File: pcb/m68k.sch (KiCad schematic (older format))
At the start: 120 parts, among them J1 USB_B_Micro, J2 Mini-DIN-6, J4 DB15_Male_HighDensity, J5 FTSH-105-01-L-DV-K, J6 FTSH-105-01-L-DV-K, J7 FTSH-105-01-L-DV-K, J8 Micro_SD_Card, U1 93LC56, U10 25LCxxx, U11 TXB0108DQSR, U12 TXB0108DQSR, U13 iCE40-HX4K-TQ144, U14 ADV7125KSTZ50, U15 74LVC1G17, U16 LD1117S33TR_SOT223, U17 LD1117S12TR_SOT223, U18 ATL431BQDBZR, U2 68000D, U3 FT2232H, U4 TXB0108DQSR, U5 TXB0108DQSR, U6 TXB0108DQSR, U7 SN74LVC8T245PWR, U8 SN74LVC8T245PWR, U9 AS6C1616, X1 ASV-12.000MHz

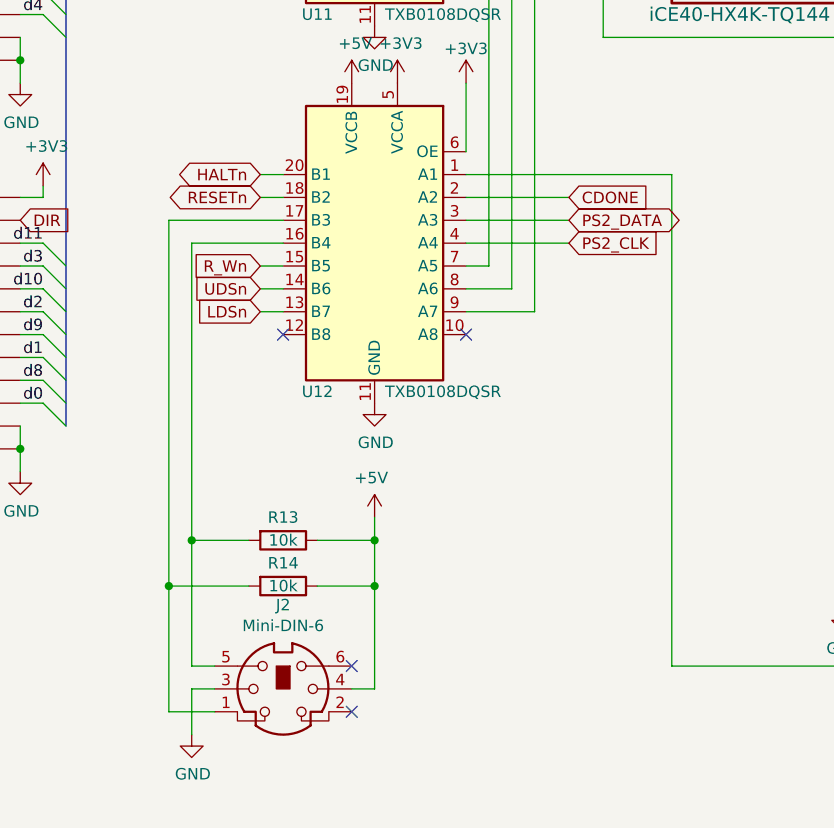
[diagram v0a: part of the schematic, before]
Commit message: Home
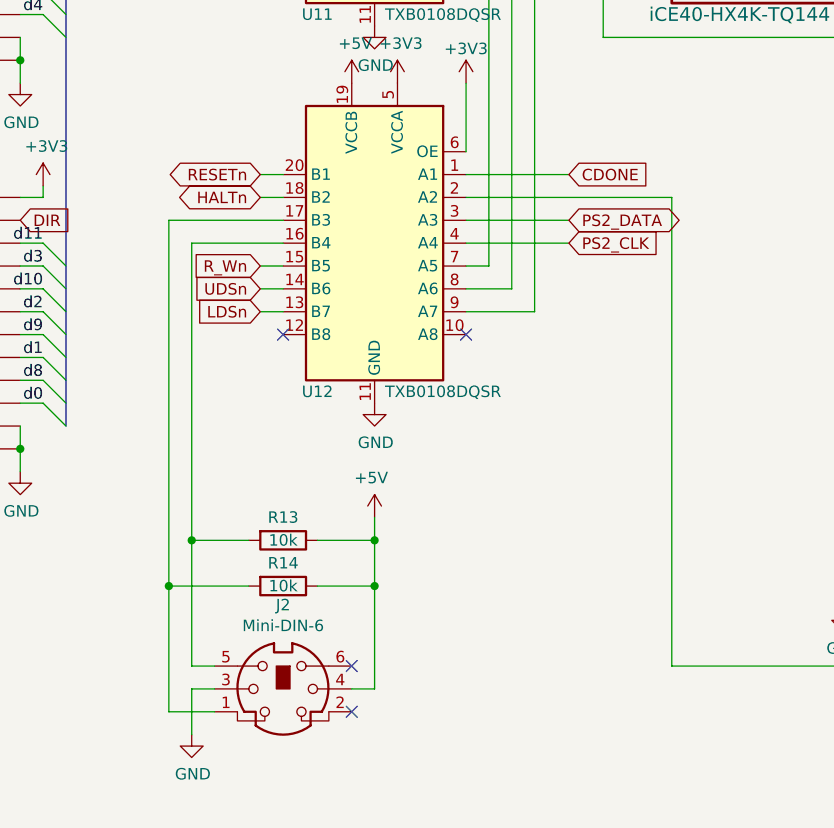
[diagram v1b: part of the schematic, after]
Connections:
- net CDONE: now also U12.1 (A1); no longer U12.2 (A2)
- net HALTn: now also U12.18 (B2); no longer U12.20 (B1)
- net RESETn: now also U12.20 (B1); no longer U12.18 (B2)
- net at U13.60 (IOB_95): now also U12.2 (A2); no longer U12.1 (A1)
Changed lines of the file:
@@
 Connection ~ 1550 14950
 Wire Wire Line
-	7050 8250 6950 8250
+	7050 8150 6950 8150
 Wire Wire Line
 	6950 7000 7050 7000
@@
 	1    0    0    -1
 $EndComp
-Text GLabel 6950 8250 0    50   BiDi ~ 0
+Text GLabel 6950 8150 0    50   BiDi ~ 0
 RESETn
-Text GLabel 8300 8250 2    50   Input ~ 0
+Text GLabel 8300 8150 2    50   Input ~ 0
 CDONE
 $Comp
@@
 Wire Wire Line
 	3400 8950 3500 8950
-Text GLabel 6950 8150 0    50   BiDi ~ 0
+Text GLabel 6950 8250 0    50   BiDi ~ 0
 HALTn
 Wire Wire Line
@@
 NoConn ~ 7050 8850
 Wire Wire Line
-	6950 8150 7050 8150
+	6950 8250 7050 8250
 Wire Wire Line
 	6550 8350 7050 8350
@@
 	7850 8350 8300 8350
 Wire Wire Line
-	7850 8250 8300 8250
-Wire Wire Line
-	7850 8150 8750 8150
+	7850 8150 8300 8150
 Wire Wire Line
-	8750 8150 8750 10300
+	7850 8250 8750 8250
 Wire Wire Line
 	8750 10300 12150 10300
@@
 Wire Wire Line
 	12150 9750 13100 9750
+Wire Wire Line
+	8750 8250 8750 10300
 Wire Bus Line
 	18600 2100 18600 2800

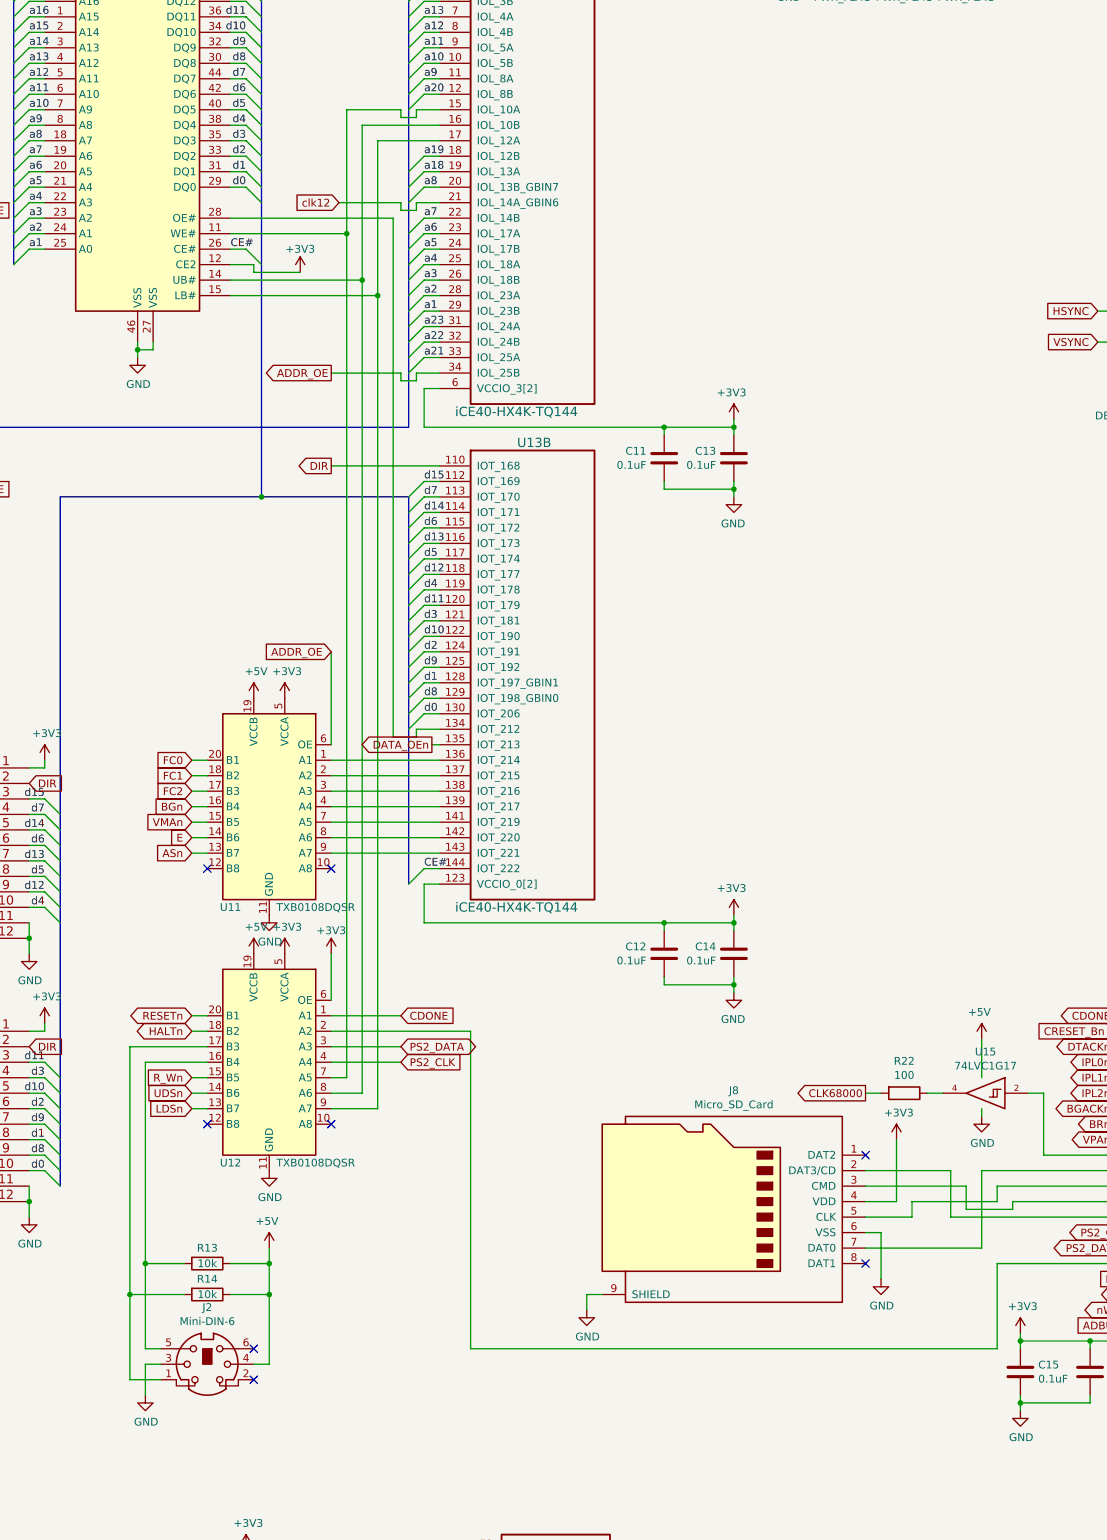
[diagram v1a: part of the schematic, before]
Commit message: I finally broke something
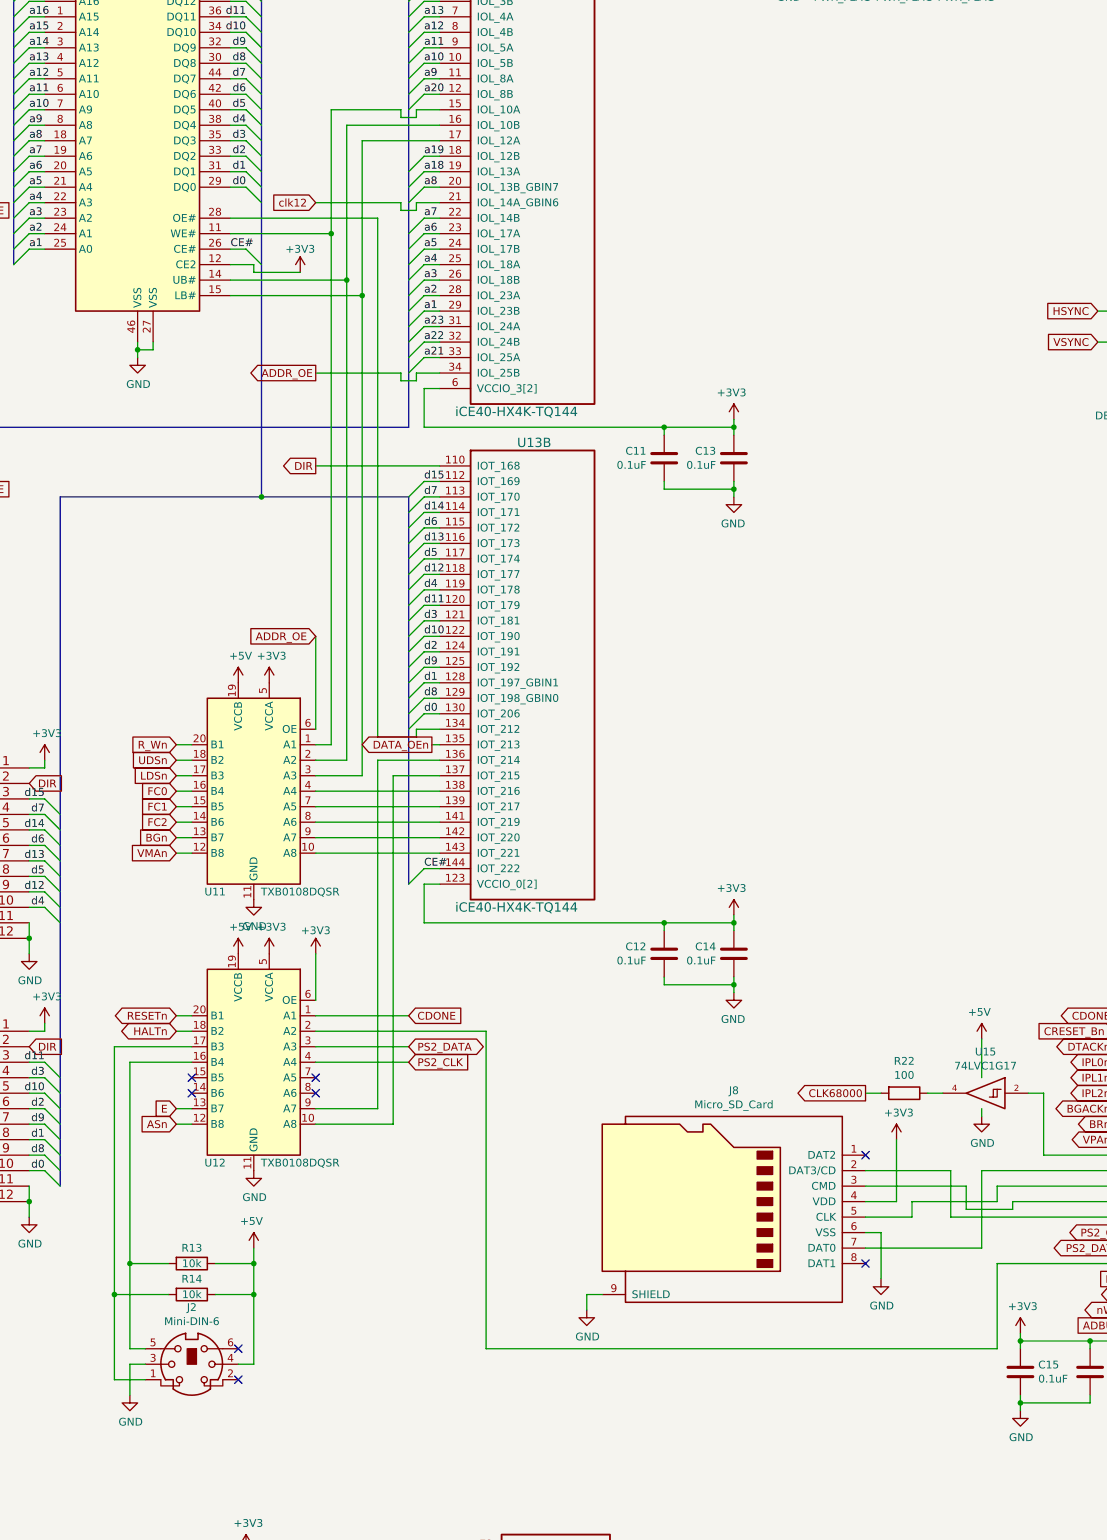
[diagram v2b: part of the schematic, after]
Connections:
- net ASn: now also U12.12 (B8); no longer U11.13 (B7)
- net BGn: now also U11.13 (B7); no longer U11.16 (B4)
- net E: now also U12.13 (B7); no longer U11.14 (B6)
- net FC0: now also U11.16 (B4); no longer U11.20 (B1)
- net FC1: now also U11.15 (B5); no longer U11.18 (B2)
- net FC2: now also U11.14 (B6); no longer U11.17 (B3)
- net LDSn: now also U11.17 (B3); no longer U12.13 (B7)
- net R_Wn: now also U11.20 (B1); no longer U12.15 (B5)
- net UDSn: now also U11.18 (B2); no longer U12.14 (B6)
- net VMAn: now also U11.12 (B8); no longer U11.15 (B5)
- net at U13.136 (IOT_214): now also U12.9 (A7); no longer U11.1 (A1)
- net at U13.137 (IOT_215): now also U12.10 (A8); no longer U11.2 (A2)
- net at U13.138 (IOT_216): now also U11.4 (A4); no longer U11.3 (A3)
- net at U13.139 (IOT_217): now also U11.7 (A5); no longer U11.4 (A4)
- net at U13.141 (IOT_219): now also U11.8 (A6); no longer U11.7 (A5)
- net at U13.142 (IOT_220): now also U11.9 (A7); no longer U11.8 (A6)
- net at U13.143 (IOT_221): now also U11.10 (A8); no longer U11.9 (A7)
- net at U13.15 (IOL_10A), U9.11 (WE#): now also U11.1 (A1); no longer U12.7 (A5)
- net at U13.16 (IOL_10B), U9.14 (UB#): now also U11.2 (A2); no longer U12.8 (A6)
- net at U13.17 (IOL_12A), U9.15 (LB#): now also U11.3 (A3); no longer U12.9 (A7)
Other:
- moved on the sheet: J2, R13, R14, U11, U12

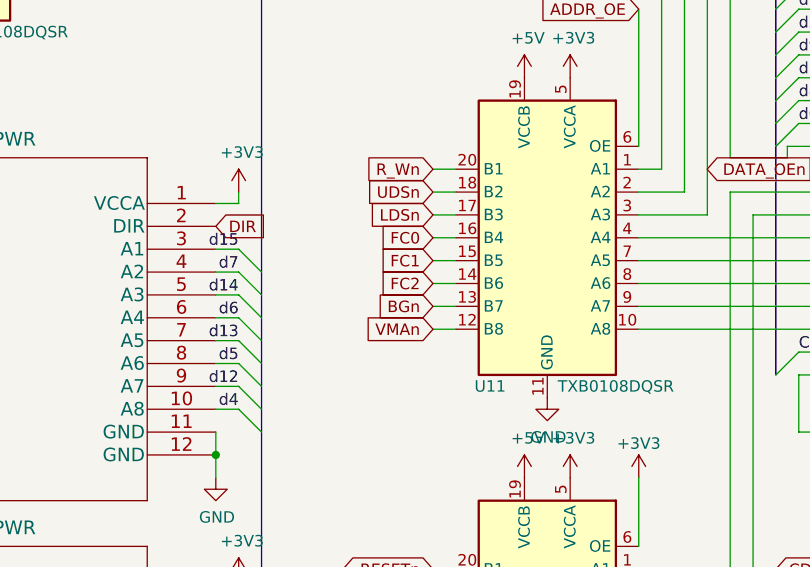
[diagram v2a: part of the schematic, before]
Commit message: Fin
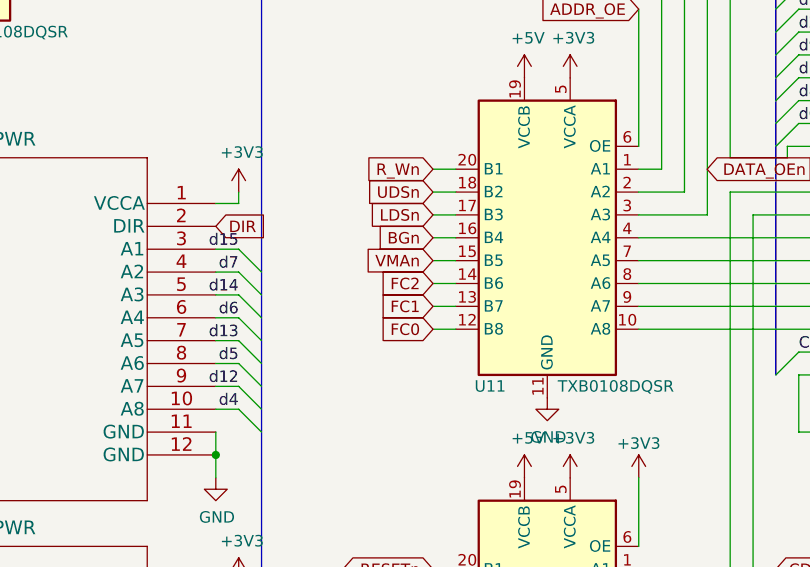
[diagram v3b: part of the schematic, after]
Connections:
- net BGn: now also U11.16 (B4); no longer U11.13 (B7)
- net FC0: now also U11.12 (B8); no longer U11.16 (B4)
- net FC1: now also U11.13 (B7); no longer U11.15 (B5)
- net VMAn: now also U11.15 (B5); no longer U11.12 (B8)
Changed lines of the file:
@@
 Connection ~ 1550 14950
 Wire Wire Line
-	6950 7100 6850 7100
-Wire Wire Line
-	6850 7000 6950 7000
+	6950 6800 6850 6800
+Wire Wire Line
+	6850 6700 6950 6700
 Text GLabel 12900 8950 0    50   Output ~ 0
 VPAn
-Text GLabel 6850 7100 0    50   Input ~ 0
+Text GLabel 6850 6800 0    50   Input ~ 0
 VMAn
 Text GLabel 12900 8850 0    50   Output ~ 0
 BRn
-Text GLabel 6850 7000 0    50   Input ~ 0
+Text GLabel 6850 6700 0    50   Input ~ 0
 BGn
 Text GLabel 12900 8750 0    50   Output ~ 0
@@
 	6850 6900 6950 6900
 Wire Wire Line
-	6950 6800 6850 6800
+	6950 7000 6850 7000
 Text GLabel 12900 8650 0    50   Output ~ 0
 IPL2n
@@
 IPL0n
 Wire Wire Line
-	6950 6700 6850 6700
+	6950 7100 6850 7100
 Text GLabel 12900 8350 0    50   Output ~ 0
 DTACKn
@@
 Wire Wire Line
 	14100 4000 13850 4000
-Text GLabel 6850 6700 0    50   Input ~ 0
+Text GLabel 6850 7100 0    50   Input ~ 0
 FC0
-Text GLabel 6850 6800 0    50   Input ~ 0
+Text GLabel 6850 7000 0    50   Input ~ 0
 FC1
 Text GLabel 6850 6900 0    50   Input ~ 0
